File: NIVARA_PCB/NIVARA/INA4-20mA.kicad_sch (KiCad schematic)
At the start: 0 parts

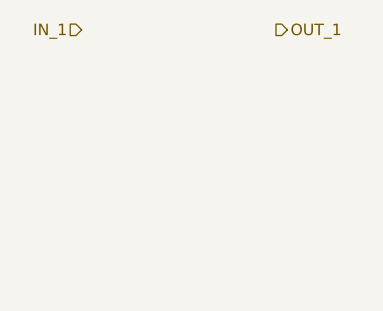
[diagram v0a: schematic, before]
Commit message: avance
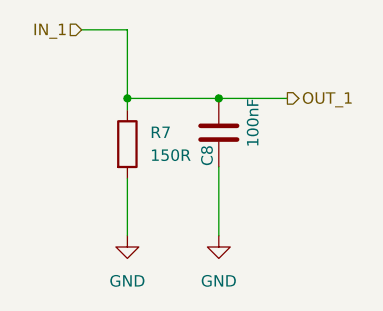
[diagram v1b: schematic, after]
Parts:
- added C8: 100nF, PCM_Capacitor_SMD_AKL:C_0603_1608Metric, symbol PCM_Capacitor_AKL:C_0603
- added R7: 150R, symbol Device:R
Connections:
- net IN_1: now also C8.2, R7.1
- new net GND: C8.1, R7.2
